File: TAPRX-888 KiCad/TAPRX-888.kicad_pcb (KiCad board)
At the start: 6 copper layers, 76 x 100 mm, 222 parts, among them J1 CONN_SMA_JACK_RA, J10 U.FL-R, J11 Conn_JTAG10-mini, J2 CONN_SMA_JACK_RA, J3 CONN_SMA_JACK_RA, J4 CONN_SMA_JACK_RA, J5 USB-3.0, J6 Conn_01x03, J7 Conn_01x03, J8 Conn_01x03, J9 Conn_01x03, Q1 PMOS Si2343DS, Q2 MMBT3904, Q3 PMOS Si2343DS, U1 AP2114H-3.3TRG1, U10 XO-19.2MHZ, U11 CYUSB3014-BZXCT, U14 LP5907MFX-3.3, U16 TLV3501, U18 NC7SV157, U19 74LVC2G14, U2 AP2114H-3.3TRG1, U20 Si5351A, U21 NC7SV157, U22 SN65LVDS1, U3 AP2114H-3.3TRG1, U4 LP5907MFX-3.3, U5 UMW AMS1117-1.2, U6 AD8370, U7 TVS-SP3011, U8 LTC2208CUP_PBF, U9 MX25L3233FM2I, X1 TCXO-27M

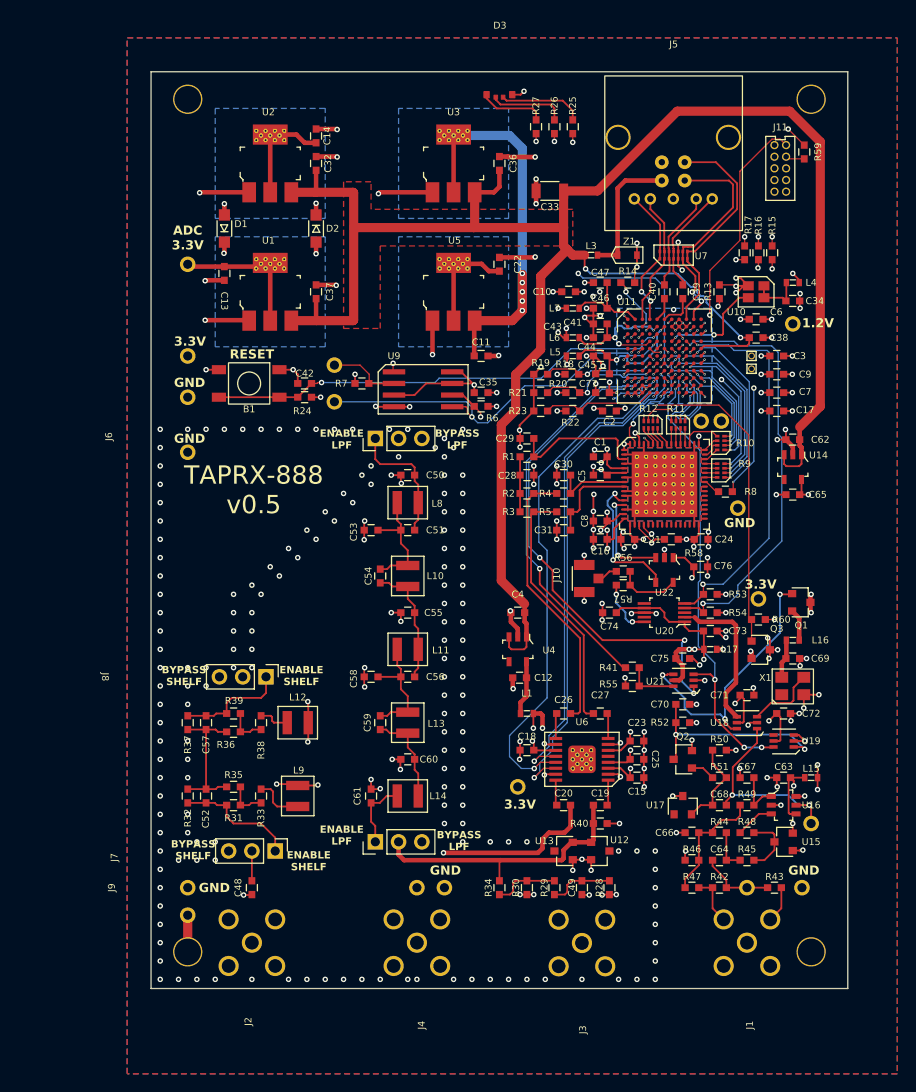
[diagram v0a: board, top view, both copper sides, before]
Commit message: proper update
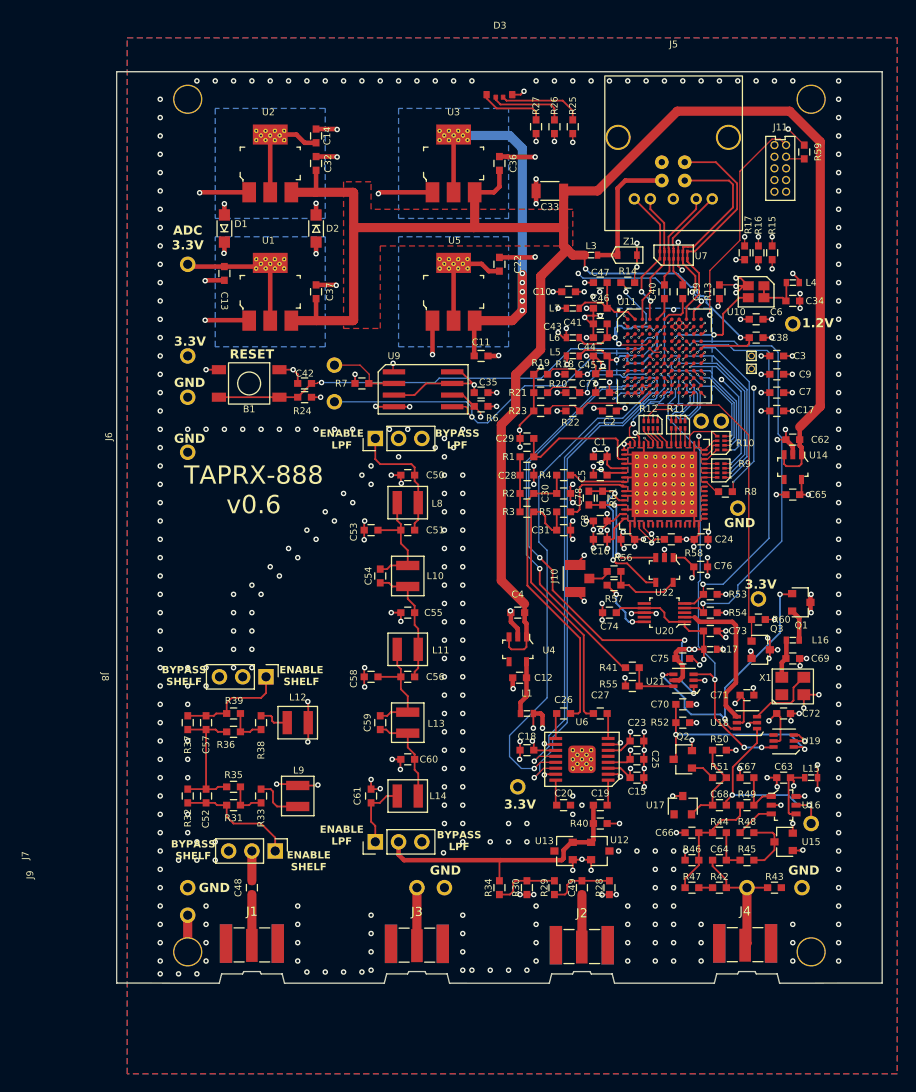
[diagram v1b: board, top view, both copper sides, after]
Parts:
- added C78: C-8.2p-0603, TIS_Footprints:PAD_0603, F.Cu at (147.8, 96.5)
- added G***: LOGO, TIS_Footprints:HamSCI-25mm, B.Cu at (118.5, 121.0)
- added R61: R-100-0603, TIS_Footprints:PAD_0603, F.Cu at (149.2, 96.5)
- J1, J2, J3, J4: value CONN_SMA_JACK_RA -> CONN_SMA_JACK_EDGE_JLC_With_Nut; footprint TIS_Footprints:SMA-RA-Jack -> TIS_Footprints:SMA_Jack_EdgeMount_JLC_With_Nut
- U8: value LTC2208CUP_PBF -> LTC2208CUP#PBF
- moved J1 54.0 mm to (111.0, 145.4), turned to 180 degrees
- moved J2 36.0 mm to (147.0, 145.6), turned to 180 degrees
- moved J4 35.8 mm to (164.8, 145.4), turned to 180 degrees
- moved J3 18.0 mm to (129.0, 145.4), turned to 180 degrees
- moved C30 2.00 mm to (145.0, 96.0), turned to 0 degrees
- moved R4 2.00 mm to (145.0, 94.0)
- moved R56 1.00 mm to (150.5, 104.5)
- moved R57 1.00 mm to (150.5, 106.0)
- moved J10 0.99 mm to (147.0, 105.3)
- turned C31 to 0 degrees
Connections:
- C30 pad 1: Net-(U8-AIN+) -> Net-(C26-Pad2)
- C31 pad 1: Net-(U8-AIN-) -> Net-(C27-Pad2)
- J1 pad 1: /Clock/EXT_REF_IN -> /Front_End_Filter/RF_IN
- J2 pad 1: /Front_End_Filter/RF_IN -> /Front_End_Filter/RF_ATTEN__IN
- J3 pad 1: /Front_End_Filter/RF_ATTEN__IN -> Net-(J3-In)
- J4 pad 1: Net-(J4-In) -> /Clock/EXT_REF_IN
- TP1 pad 1: Net-(J4-In) -> Net-(J3-In)
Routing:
- net GND: track 268.8 -> 242.0 mm, vias 326 -> 453
- net Net-(J3-In): track 0.00 -> 6.32 mm
- net Net-(J4-In): track 6.00 -> 0.00 mm
- net Net-(C27-Pad2): track 27.9 -> 31.2 mm
- net /SAMPLE_CLK_N: track 10.9 -> 13.7 mm
- net /SAMPLE_CLK_P: track 15.5 -> 17.9 mm
- net Net-(U8-AIN+): track 8.37 -> 6.16 mm
- net Net-(C26-Pad2): track 30.1 -> 32.1 mm
- net Net-(U8-AIN-): track 10.2 -> 8.56 mm
- net Net-(R56-Pad2): track 6.95 -> 7.95 mm
- net Net-(J10-In): track 1.85 -> 2.51 mm
- net /Front_End_Filter/RF_ATTEN__IN: track 6.32 -> 5.73 mm, vias 1 -> 0
- net /Front_End_Filter/RF_IN: track 6.42 -> 6.16 mm, vias 1 -> 0
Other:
- board size 76 x 100 mm -> 83.5 x 99.4 mm
- board text added: "Commit: ${GIT_HASH}"
- board text added: "Note: SMA connectors extend 0.6mm from board edge, 99.4mm + 0.6mm = 100mm"
- board text added: "TAPRX-888 v0.6"
- board text removed: "TAPRX-888 v0.5"
